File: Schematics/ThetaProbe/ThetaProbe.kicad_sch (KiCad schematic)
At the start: 15 parts, among them J1 BME280, J2 Relay_Module, J3 LED_Connection, J4 LED_Alive, J5 1-Wire CH1, J6 1-Wire CH2, J7 Power, U1 ESP32-DevKitC

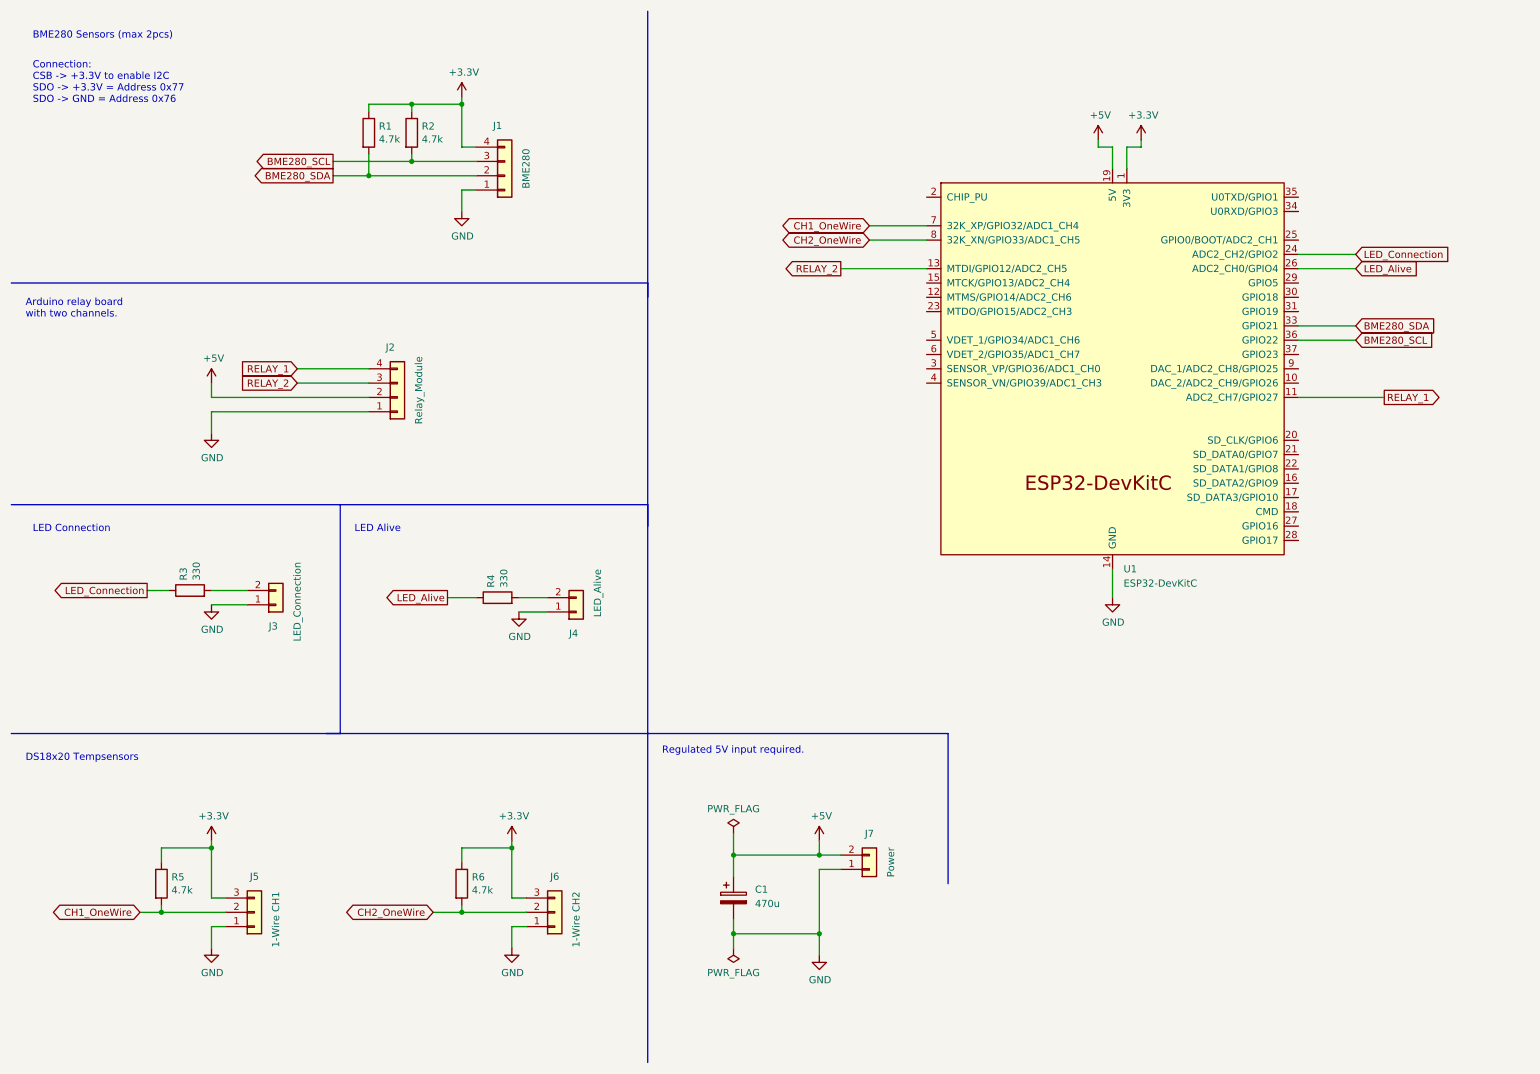
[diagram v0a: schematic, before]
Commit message: Debug LED added.
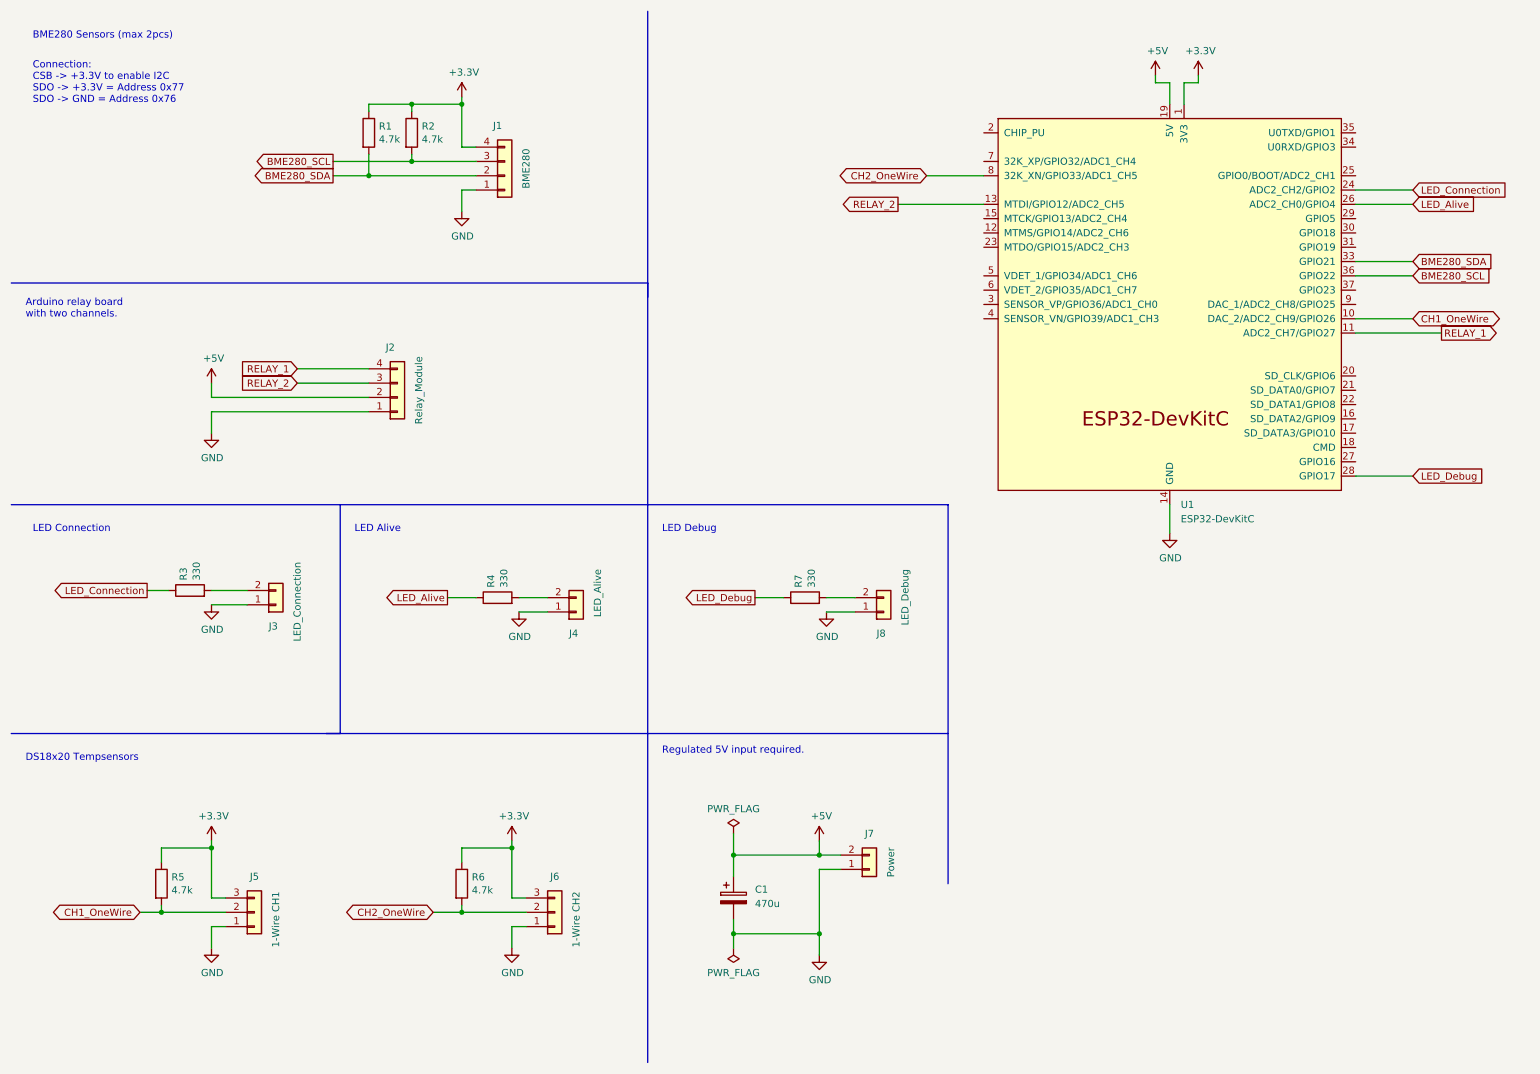
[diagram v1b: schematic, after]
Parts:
- added J8: LED_Debug, Connector_Molex:Molex_KK-254_AE-6410-02A_1x02_P2.54mm_Vertical, symbol Connector_Generic:Conn_01x02
- added R7: 330, Resistor_THT:R_Axial_DIN0207_L6.3mm_D2.5mm_P7.62mm_Horizontal, symbol Device:R
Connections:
- net CH1_OneWire: now also U1.10 (DAC_2/ADC2_CH9/GPIO26); no longer U1.7 (32K_XP/GPIO32/ADC1_CH4)
- net GND: now also J8.1 (Pin_1)
- net LED_Debug: now reaches U1.28 (GPIO17)
- net LED_Debug: now also R7.1
- new net: J8.2 (Pin_2), R7.2
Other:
- note added: "LED Debug"
- moved on the sheet: U1
